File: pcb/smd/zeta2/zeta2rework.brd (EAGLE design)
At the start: 121.6 x 87.6 mm, 114 parts, among them IC1 MAX6520, IC2 L293DD, IC3 L293DD, Q12 8MHz, U1 MPU-6050, U2 INA219, U4 INA219, U5 DS18B20U+

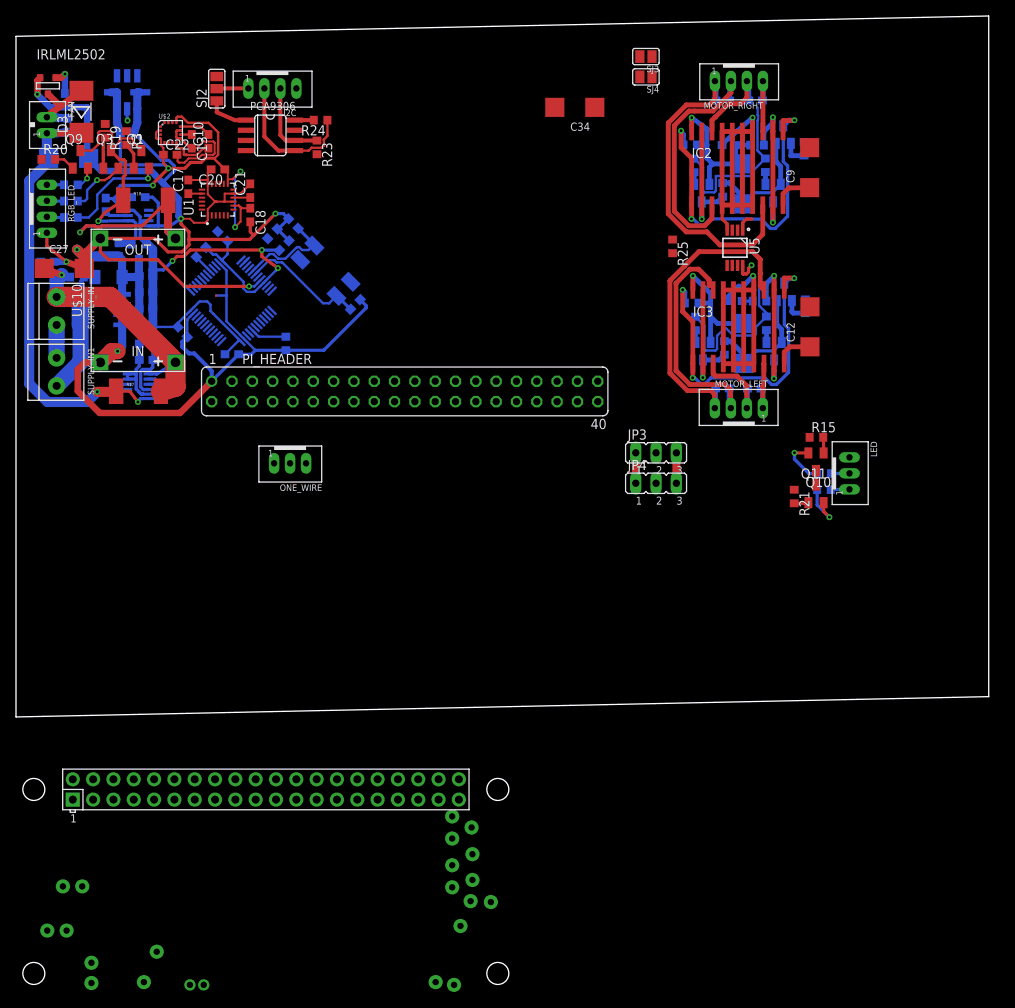
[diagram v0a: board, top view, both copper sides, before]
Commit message: added hall effect sensor
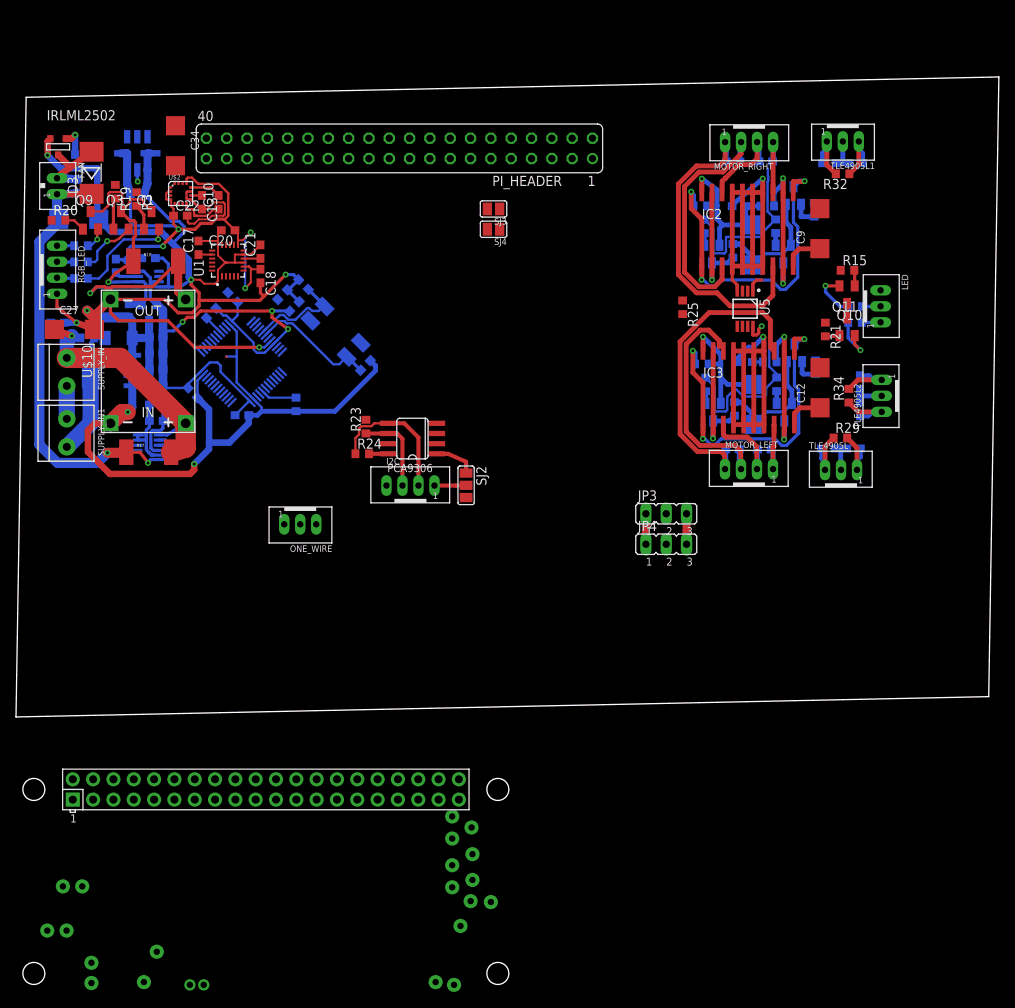
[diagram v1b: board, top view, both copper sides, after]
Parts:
- added C19, C30, C32, C35, C42, C44: 4.7nF, rcl:C0603
- added R29, R32, R34: 1.2k, rcl:R0603
- added TLE4905L, TLE4905L1, TLE4905L2: JST-PH_3-PIN_HEADER, srg:JST_B3B-PH_HEADER
- moved SJ2 58.6 mm to (55.0, 23.9), turned to 270 degrees
- moved I2C 52.7 mm to (48.1, 23.8), turned to 0 degrees
- moved C34 50.1 mm to (18.7, 66.3), turned to 270 degrees
- moved R24 42.0 mm to (42.0, 27.8), turned to 0 degrees
- moved PCA9306 41.8 mm to (48.3, 29.7), turned to 90 degrees
- moved R23 35.4 mm to (42.5, 31.2), turned to 90 degrees
- moved PI_HEADER 30.4 mm to (46.7, 66.0), turned to 180 degrees
- moved SJ4 26.9 mm to (58.4, 55.9)
- moved SJ3 26.9 mm to (58.4, 58.4)
- moved Q10 21.2 mm to (102.6, 47.7)
- moved Q11 21.2 mm to (102.6, 43.7)
- moved R15 21.2 mm to (102.7, 50.7)
- moved R16 21.2 mm to (103.6, 44.2)
- moved R4 21.2 mm to (103.6, 46.2)
- moved LED 21.2 mm to (106.8, 46.3)
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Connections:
- new net HALL_1: C30.2, R29.1, TLE4905L.P3
- new net HALL_2: C35.2, R32.1, TLE4905L1.P3
- new net HALL_3: C44.2, R34.1, TLE4905L2.P3
- net +5V: now also C19.1, C32.1, C42.1, R29.2, R32.2, R34.2, TLE4905L.P1, TLE4905L1.P1, TLE4905L2.P1
- net GND: now also C19.2, C30.1, C32.2, C35.1, C42.2, C44.1, TLE4905L.P2, TLE4905L1.P2, TLE4905L2.P2
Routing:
- net +5V: track 75.2 -> 97.5 mm
- net GND: track 431.3 -> 443.9 mm, vias 9 -> 10
- net HALL_3: track 0.00 -> 7.48 mm
- net HALL_2: track 0.00 -> 7.46 mm
- net HALL_1: track 0.00 -> 7.28 mm
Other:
- board size 121.6 x 87.6 mm -> 122.9 x 80 mm
